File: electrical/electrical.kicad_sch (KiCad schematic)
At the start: 0 parts

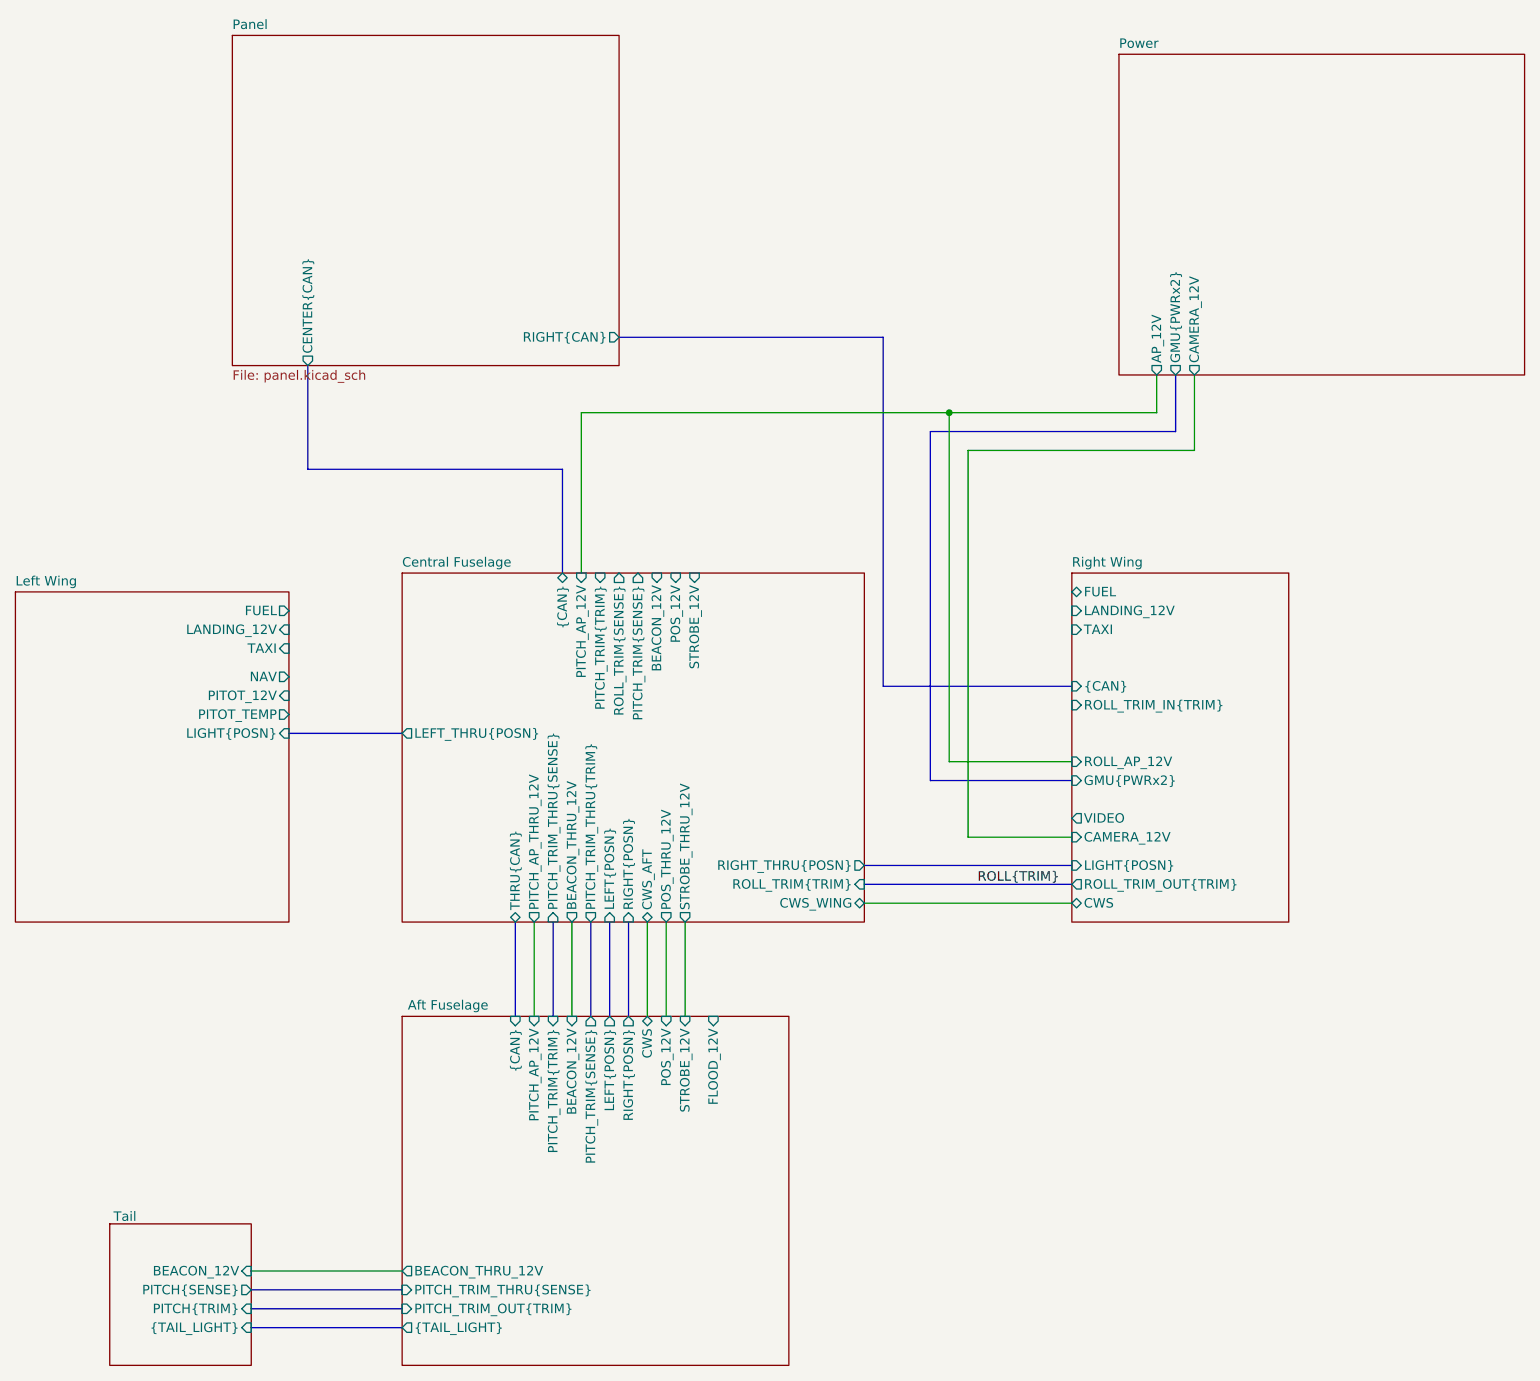
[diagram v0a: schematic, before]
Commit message: 🎮 Working on electrical schematic
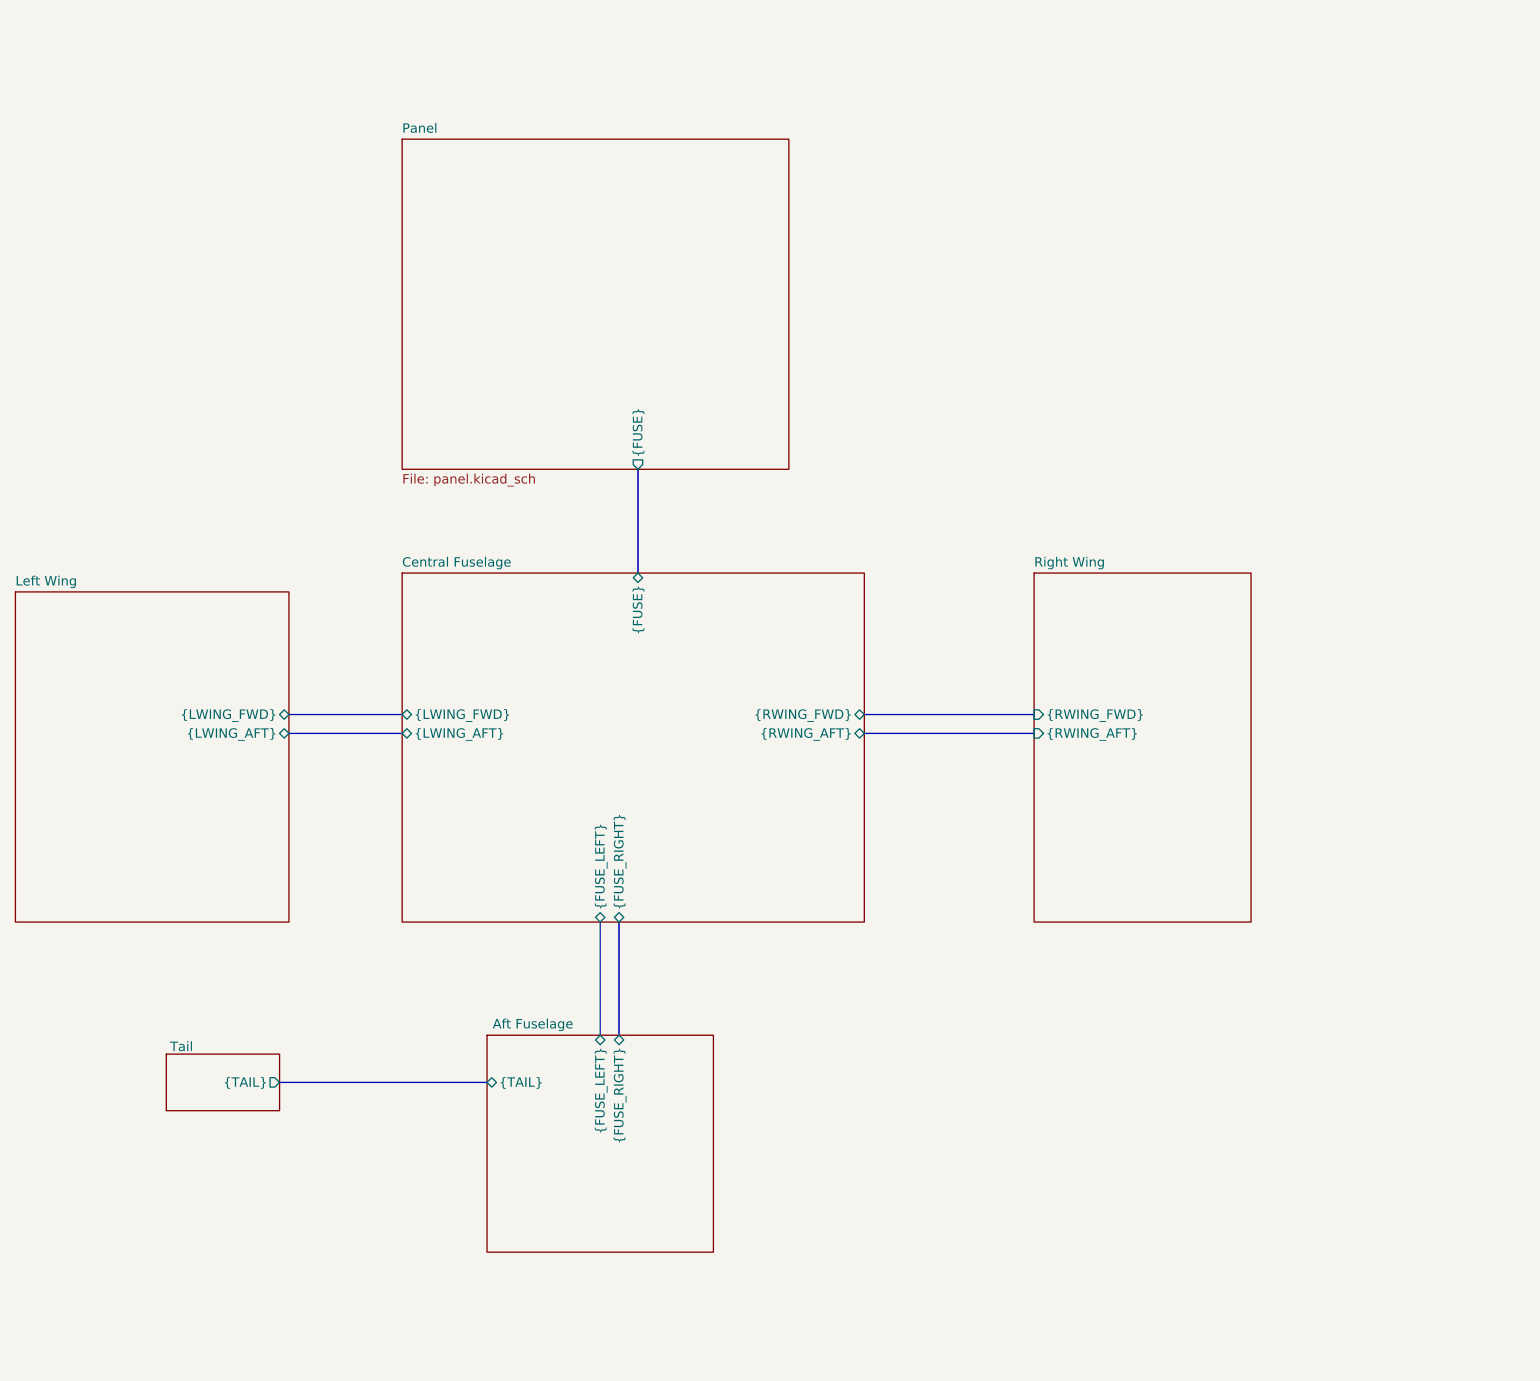
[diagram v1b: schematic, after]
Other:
- removed sheet Power
- sheet Aft Fuselage ports: added {FUSE_LEFT}, {FUSE_RIGHT}, {TAIL}; removed BEACON_12V, BEACON_THRU_12V, CWS, FLOOD_12V, LEFT{POSN}, PITCH_AP_12V, PITCH_TRIM_OUT{TRIM}, PITCH_TRIM_THRU{SENSE}, PITCH_TRIM{SENSE}, PITCH_TRIM{TRIM}, POS_12V, RIGHT{POSN}, STROBE_12V, {CAN}, {TAIL_LIGHT}
- sheet Central Fuselage ports: added {FUSE_LEFT}, {FUSE_RIGHT}, {FUSE}, {LWING_AFT}, {LWING_FWD}, {RWING_AFT}, {RWING_FWD}; removed BEACON_12V, BEACON_THRU_12V, CWS_AFT, CWS_WING, LEFT_THRU{POSN}, LEFT{POSN}, PITCH_AP_12V, PITCH_AP_THRU_12V, PITCH_TRIM_THRU{SENSE}, PITCH_TRIM_THRU{TRIM}, PITCH_TRIM{SENSE}, PITCH_TRIM{TRIM}, POS_12V, POS_THRU_12V, RIGHT_THRU{POSN}, RIGHT{POSN}, ROLL_TRIM{SENSE}, ROLL_TRIM{TRIM}, STROBE_12V, STROBE_THRU_12V, THRU{CAN}, {CAN}
- sheet Left Wing ports: added {LWING_AFT}, {LWING_FWD}; removed FUEL, LANDING_12V, LIGHT{POSN}, NAV, PITOT_12V, PITOT_TEMP, TAXI
- sheet Panel ports: added {FUSE}; removed CENTER{CAN}, RIGHT{CAN}
- sheet Right Wing ports: added {RWING_AFT}, {RWING_FWD}; removed CAMERA_12V, CWS, FUEL, GMU{PWRx2}, LANDING_12V, LIGHT{POSN}, ROLL_AP_12V, ROLL_TRIM_IN{TRIM}, ROLL_TRIM_OUT{TRIM}, TAXI, VIDEO, {CAN}
- sheet Tail ports: added {TAIL}; removed BEACON_12V, PITCH{SENSE}, PITCH{TRIM}, {TAIL_LIGHT}
